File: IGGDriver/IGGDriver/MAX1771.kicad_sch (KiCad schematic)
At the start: 15 parts, among them Q129 NMOS, U17 MAX1771xSA

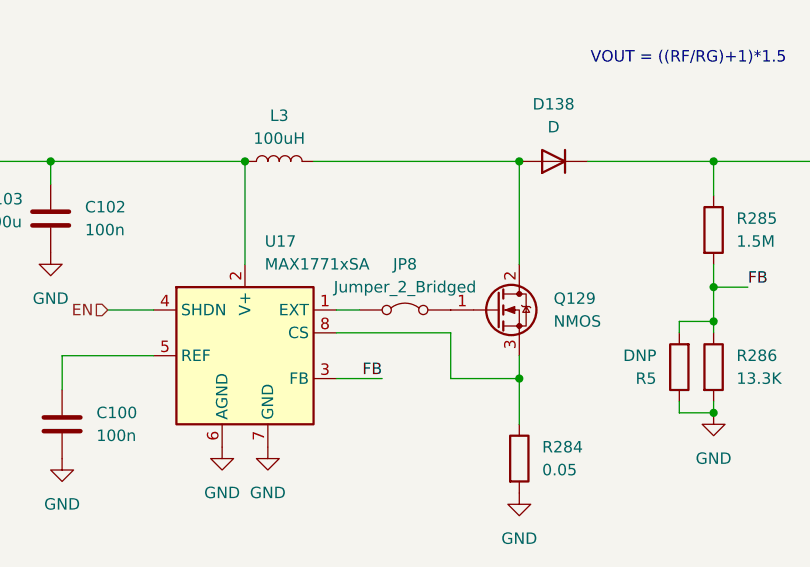
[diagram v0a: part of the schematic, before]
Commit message: Commit to xfer to other computer
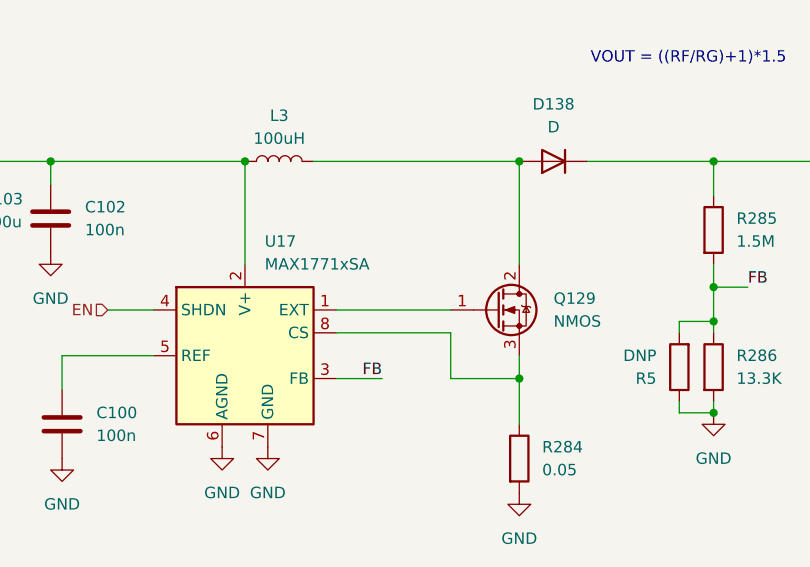
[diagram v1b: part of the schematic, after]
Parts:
- removed JP8: Jumper_2_Bridged, Jumper:SolderJumper-2_P1.3mm_Bridged_RoundedPad1.0x1.5mm, symbol Jumper:Jumper_2_Bridged
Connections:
- net at Q129.1 (G): now also U17.1 (EXT)
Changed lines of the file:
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@@
 	(wire
 		(pts
-			(xy 148.59 67.31) (xy 151.13 67.31)
+			(xy 148.59 67.31) (xy 161.29 67.31)
 		)
 		(stroke
@@
 					(unit 1)
 				)
-			)
-		)
-	)
-	(symbol
-		(lib_id "Jumper:Jumper_2_Bridged")
-		(at 156.21 67.31 0)
-		(unit 1)
-		(exclude_from_sim yes)
-		(in_bom yes)
-		(on_board yes)
-		(dnp no)
-		(fields_autoplaced yes)
-		(property "Reference" "JP8"
-			(at 156.21 62.23 0)
-			(effects
-				(font
-					(size 1.27 1.27)
-				)
-			)
-		)
-		(property "Value" "Jumper_2_Bridged"
-			(at 156.21 64.77 0)
-			(effects
-				(font
-					(size 1.27 1.27)
-				)
-			)
-		)
-		(property "Footprint" "Jumper:SolderJumper-2_P1.3mm_Bridged_RoundedPad1.0x1.5mm"
-			(at 156.21 67.31 0)
-			(effects
-				(font
-					(size 1.27 1.27)
-				)
-				(hide yes)
-			)
-		)
-		(property "Datasheet" "~"
-			(at 156.21 67.31 0)
-			(effects
-				(font
-					(size 1.27 1.27)
-				)
-				(hide yes)
-			)
-		)
-		(property "Description" "Jumper, 2-pole, closed/bridged"
-			(at 156.21 67.31 0)
-			(effects
-				(font
-					(size 1.27 1.27)
-				)
-				(hide yes)
-			)
-		)
-		(property "LCSC" ""
-			(at 156.21 67.31 0)
-			(effects
-				(font
-					(size 1.27 1.27)
-				)
-				(hide yes)
-			)
-		)
-		(pin "1"
-		)
-		(pin "2"
-		)
-		(instances
-			(project "IGGDriver"
-				(path "/42dcdc8e-b1dc-4d4c-b3c7-96447ce841be/ad819f5f-9558-4b19-bdf0-0c64035fd7cc"
-					(reference "JP8")
-					(unit 1)
-				)

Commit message: RTM
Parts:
- L3: LCSC C408533 -> C408533
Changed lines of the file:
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@@
 			)
 		)
-		(property "LCSC" "    C408533"
+		(property "LCSC" " C408533"
 			(at 142.24 50.8 90)
 			(effects

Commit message: Added mechanicDDDDl stuff, case, etc
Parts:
- L3: LCSC C408533 -> C408533
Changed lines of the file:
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@@
 			)
 		)
-		(property "LCSC" " C408533"
+		(property "LCSC" "C408533"
 			(at 142.24 50.8 90)
 			(effects
